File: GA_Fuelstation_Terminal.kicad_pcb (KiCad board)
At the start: 2 copper layers, 136.6 x 58.4 mm, 36 parts, among them IC1 ESP32-S3-WROOM-1, J1 Conn_01x08_Pin, J10 Screw_Terminal_01x02, J2 Conn_01x05_Pin, J5 Conn_01x02_Pin, J6 Screw_Terminal_01x02, J7 Screw_Terminal_01x02, J98 Conn_01x07_Socket, J99 Conn_ARM_JTAG_SWD_20, Q1 2N7002, Q2 2N7002, Q3 2N7002, U1 3V3, U2 5V

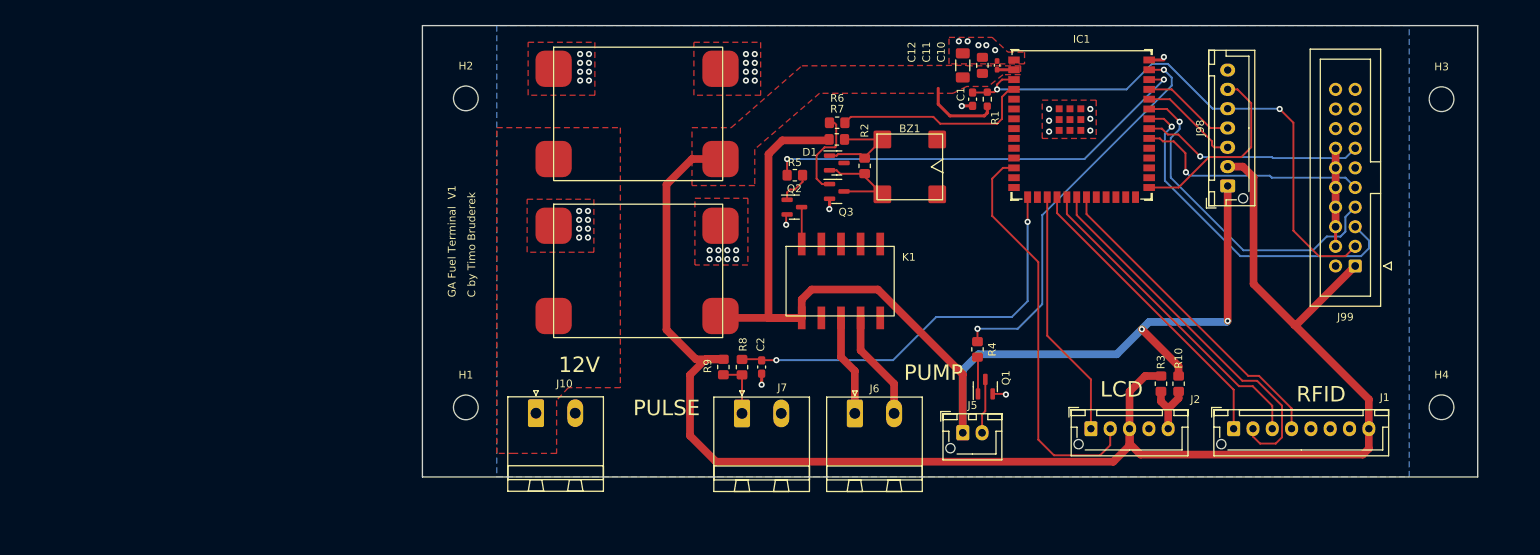
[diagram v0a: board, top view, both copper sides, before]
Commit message: LAN PHy
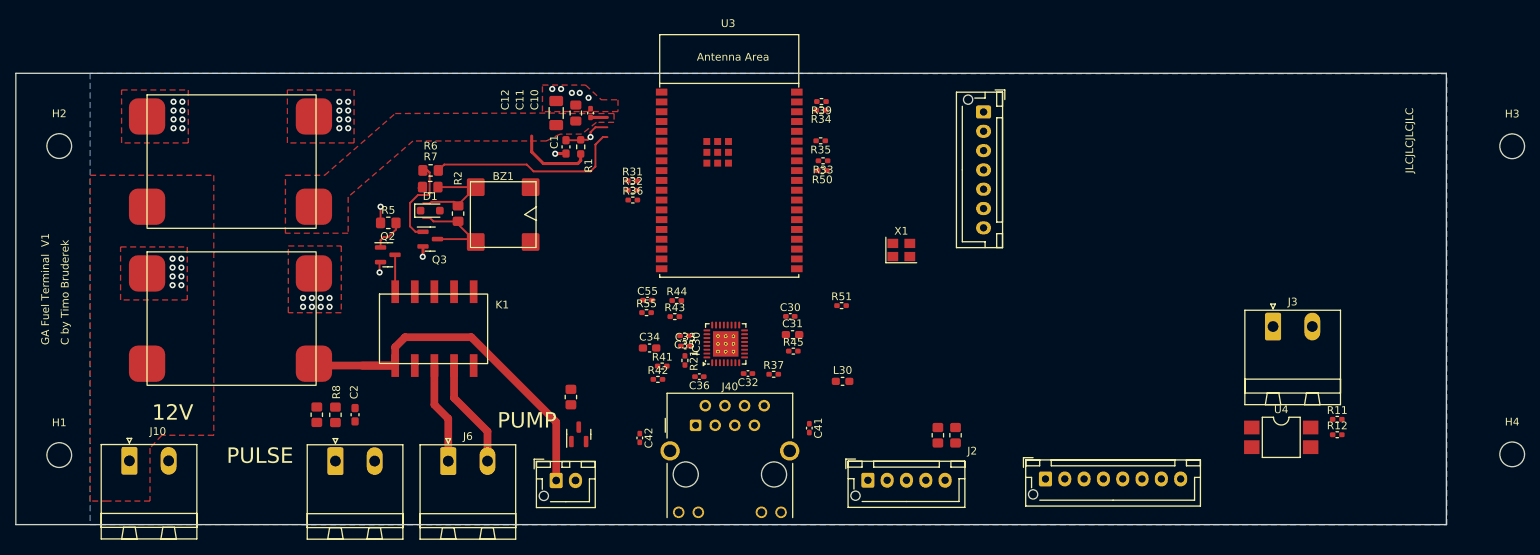
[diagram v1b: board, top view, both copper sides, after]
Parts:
- removed IC1: ESP32-S3-WROOM-1, Espressif:ESP32-S3-WROOM-1U
- removed J99: Conn_ARM_JTAG_SWD_20, Connector_IDC:IDC-Header_2x10_P2.54mm_Vertical
- added C30: 100nF, Capacitor_SMD:C_0402_1005Metric_Pad0.74x0.62mm_HandSolder, F.Cu at (164.4, 80.2)
- added C31: 10uF, Capacitor_SMD:C_0603_1608Metric_Pad1.08x0.95mm_HandSolder, F.Cu at (164.7, 82.5)
- added C32: 100nF, Capacitor_SMD:C_0402_1005Metric_Pad0.74x0.62mm_HandSolder, F.Cu at (158.9, 87.6)
- added C33: 100nF, Capacitor_SMD:C_0402_1005Metric_Pad0.74x0.62mm_HandSolder, F.Cu at (150.8, 84.0)
- added C34: 10uF, Capacitor_SMD:C_0603_1608Metric_Pad1.08x0.95mm_HandSolder, F.Cu at (146.2, 84.3)
- added C35: 100nF, Capacitor_SMD:C_0402_1005Metric_Pad0.74x0.62mm_HandSolder, F.Cu at (150.7, 82.7)
- added C36: 100nF, Capacitor_SMD:C_0402_1005Metric_Pad0.74x0.62mm_HandSolder, F.Cu at (152.6, 88.0)
- added C41: 100nF 25V, Capacitor_SMD:C_0402_1005Metric_Pad0.74x0.62mm_HandSolder, F.Cu at (166.8, 94.6)
- added C42: 100nF 25V, Capacitor_SMD:C_0402_1005Metric_Pad0.74x0.62mm_HandSolder, F.Cu at (144.9, 95.9)
- added C55: 100nF, Capacitor_SMD:C_0402_1005Metric_Pad0.74x0.62mm_HandSolder, F.Cu at (145.9, 78.1)
- added IC30: RTL8201F, Package_DFN_QFN:QFN-32-1EP_5x5mm_P0.5mm_EP3.3x3.3mm_ThermalVias, F.Cu at (156.0, 83.7)
- added J3: Screw_Terminal_01x02, Connector_Phoenix_MSTB:PhoenixContact_MSTBA_2,5_2-G-5,08_1x02_P5.08mm_Horizontal, F.Cu at (226.9, 81.5)
- added J40: RJ45_Hanrun_HR911105A_Horizontal, Connector_RJ:RJ45_Hanrun_HR911105A_Horizontal, F.Cu at (152.1, 94.3)
- added L30: HCB1608FK-501T20, Inductor_SMD:L_0603_1608Metric_Pad1.05x0.95mm_HandSolder, F.Cu at (171.1, 88.6)
- added R11: R, Resistor_SMD:R_0402_1005Metric_Pad0.72x0.64mm_HandSolder, F.Cu at (235.2, 93.5)
- added R12: R, Resistor_SMD:R_0402_1005Metric_Pad0.72x0.64mm_HandSolder, F.Cu at (235.2, 95.5)
- added R21: 2k49 1%, Resistor_SMD:R_0402_1005Metric_Pad0.72x0.64mm_HandSolder, F.Cu at (150.7, 85.9)
- added R31: 22R, Resistor_SMD:R_0402_1005Metric_Pad0.72x0.64mm_HandSolder, F.Cu at (143.9, 62.6)
- added R32: 22R, Resistor_SMD:R_0402_1005Metric_Pad0.72x0.64mm_HandSolder, F.Cu at (143.9, 63.9)
- added R33: 22R, Resistor_SMD:R_0402_1005Metric_Pad0.72x0.64mm_HandSolder, F.Cu at (168.6, 60.0)
- added R34: 22R, Resistor_SMD:R_0402_1005Metric_Pad0.72x0.64mm_HandSolder, F.Cu at (168.4, 53.5)
- added R35: 22R, Resistor_SMD:R_0402_1005Metric_Pad0.72x0.64mm_HandSolder, F.Cu at (168.3, 57.5)
- added R36: 22R, Resistor_SMD:R_0402_1005Metric_Pad0.72x0.64mm_HandSolder, F.Cu at (144.0, 65.1)
- added R37: 10K, Resistor_SMD:R_0402_1005Metric_Pad0.72x0.64mm_HandSolder, F.Cu at (162.2, 87.7)
- added R39: 22R, Resistor_SMD:R_0402_1005Metric_Pad0.72x0.64mm_HandSolder, F.Cu at (168.4, 52.4)
- added R41: 4k7, Resistor_SMD:R_0402_1005Metric_Pad0.72x0.64mm_HandSolder, F.Cu at (147.8, 86.6)
- added R42: 4k7, Resistor_SMD:R_0402_1005Metric_Pad0.72x0.64mm_HandSolder, F.Cu at (147.2, 88.3)
- added R43: 4k7, Resistor_SMD:R_0402_1005Metric_Pad0.72x0.64mm_HandSolder, F.Cu at (149.4, 80.2)
- added R44: 220R, Resistor_SMD:R_0402_1005Metric_Pad0.72x0.64mm_HandSolder, F.Cu at (149.7, 78.1)
- added R45: 4k7, Resistor_SMD:R_0402_1005Metric_Pad0.72x0.64mm_HandSolder, F.Cu at (164.8, 84.7)
- added R50: 22R, Resistor_SMD:R_0402_1005Metric_Pad0.72x0.64mm_HandSolder, F.Cu at (168.5, 61.3)
- added R51: 10k, Resistor_SMD:R_0402_1005Metric_Pad0.72x0.64mm_HandSolder, F.Cu at (171.0, 78.8)
- added R55: 4k7, Resistor_SMD:R_0402_1005Metric_Pad0.72x0.64mm_HandSolder, F.Cu at (145.8, 79.7)
- added U3: ESP32-WROVER-E, Espressif:ESP32-WROVER-E, F.Cu at (156.5, 59.4)
- added U4: EL817, Package_DIP:SMDIP-4_W7.62mm, F.Cu at (227.9, 95.8)
- added X1: ASE-xxxMHz, Crystal:Crystal_SMD_3225-4Pin_3.2x2.5mm, F.Cu at (178.7, 71.6)
- C1: value 1u -> 4u7
- C10: value 100nF / 50V -> 100nF / 50V
- D1: value D -> 1N4148; footprint Package_TO_SOT_SMD:SOT-23 -> Diode_SMD:D_SOD-323_HandSoldering
- R7: value R -> 0R
- R9: value 50k -> 68k
- moved C1 53.0 mm to (135.3, 58.2)
- moved D1 53.0 mm to (117.8, 66.5)
- moved J7 53.0 mm to (105.5, 98.9)
- moved K1 53.0 mm to (113.2, 86.5)
- moved Q3 53.0 mm to (117.8, 70.2)
- moved R1 53.0 mm to (137.2, 58.2)
- moved R2 53.0 mm to (121.4, 66.9)
- moved R4 53.0 mm to (136.0, 90.6)
- moved R7 53.0 mm to (117.8, 63.4)
- moved R8 53.0 mm to (105.5, 92.9)
- moved BZ1 53.0 mm to (127.2, 67.0)
- moved C2 53.0 mm to (108.0, 92.9)
- moved H1 53.0 mm to (69.7, 98.1)
- moved H2 53.0 mm to (69.7, 58.1)
- moved J10 53.0 mm to (78.8, 98.9)
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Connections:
- R9 pad 2: Net-(J7-Pin_1) -> IO_PUMP_PULSE
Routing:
- net +3.3V: track 221.7 -> 12.2 mm
- net +5V: track 151.6 -> 51.4 mm, vias 2 -> 0
- net EN: track 73.2 -> 6.43 mm, vias 2 -> 1
- net IO_PUMP_RELAIS: track 57.0 -> 2.09 mm, vias 2 -> 1
- net IO_PUMP_PULSE: track 53.1 -> 0.00 mm, vias 2 -> 0
- net SDA: track 52.5 -> 0.00 mm
- net IO_PUMP_LED: track 51.0 -> 0.00 mm, vias 2 -> 0
- net SCK: track 48.7 -> 0.00 mm
- net TDI: track 45.1 -> 0.00 mm, vias 1 -> 0
- net TMS: track 43.5 -> 0.00 mm, vias 1 -> 0
- net MOSI: track 42.0 -> 0.00 mm
- net MISO: track 41.8 -> 0.00 mm
- net RFID_SS: track 39.4 -> 0.00 mm
- net SCL: track 32.3 -> 0.00 mm
- net TCK: track 30.7 -> 0.00 mm, vias 1 -> 0
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- added copper zone on In1.Cu, net GND
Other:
- board size 136.6 x 58.4 mm -> 185.2 x 58.4 mm
- copper layers 2 -> 4
- board text added: "JLCJLCJLCJLC"
- board text removed: "LCD"
- board text removed: "RFID"
